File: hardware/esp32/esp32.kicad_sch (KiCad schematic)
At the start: 10 parts, among them J1 Conn_01x01, J2 Conn_01x02, J3 Conn_01x10, J6 Conn_01x01, U2 ESP32-S3-MINI-1-N8

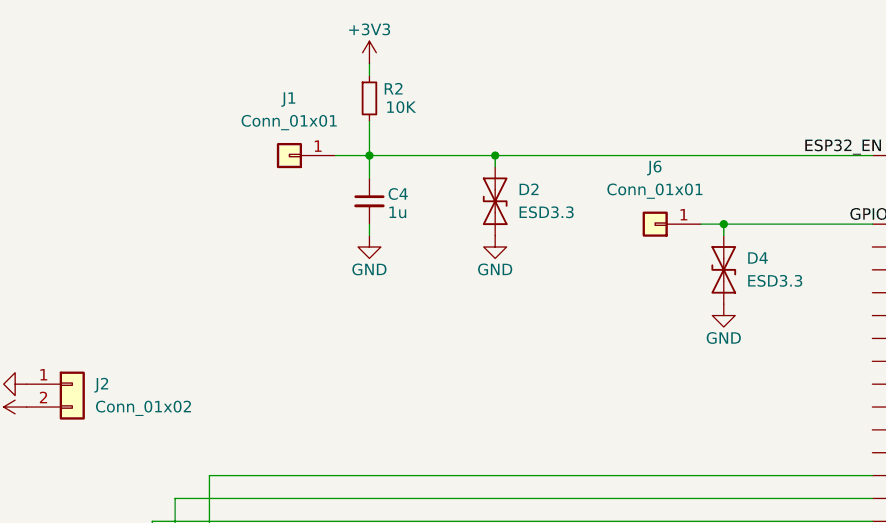
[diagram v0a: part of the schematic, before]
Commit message: wip esp32 v1
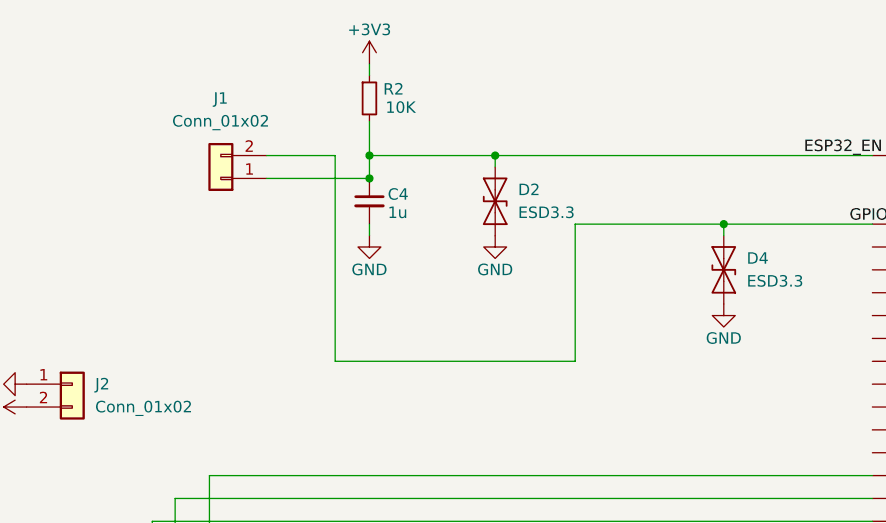
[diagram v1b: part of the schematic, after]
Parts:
- removed J1, J6: Conn_01x01, Connector_PinHeader_1.00mm:PinHeader_1x01_P1.00mm_Vertical, symbol Connector_Generic:Conn_01x01
- added J1: Conn_01x02, Connector_JST:JST_SH_BM02B-SRSS-TB_1x02-1MP_P1.00mm_Vertical, symbol Connector_Generic:Conn_01x02
- C18, C4: footprint Capacitor_SMD:C_0603_1608Metric -> Capacitor_SMD:C_0201_0603Metric
- R2: footprint Resistor_SMD:R_0402_1005Metric -> Resistor_SMD:R_0201_0603Metric
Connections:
- net ESP32_EN: now also J1.1 (Pin_1)
- net GPIO0: now also J1.2 (Pin_2)

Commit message: Revert "wip esp32 v1"
This reverts commit 4981c68ebba1a87f50308cda0493b3bcd30c48b4.
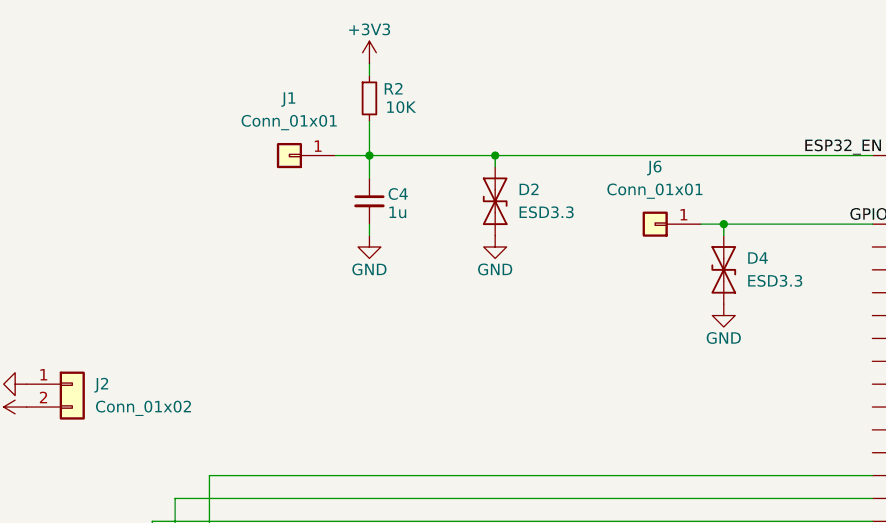
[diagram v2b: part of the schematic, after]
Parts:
- removed J1: Conn_01x02, Connector_JST:JST_SH_BM02B-SRSS-TB_1x02-1MP_P1.00mm_Vertical, symbol Connector_Generic:Conn_01x02
- added J1, J6: Conn_01x01, Connector_PinHeader_1.00mm:PinHeader_1x01_P1.00mm_Vertical, symbol Connector_Generic:Conn_01x01
- C18, C4: footprint Capacitor_SMD:C_0201_0603Metric -> Capacitor_SMD:C_0603_1608Metric
- R2: footprint Resistor_SMD:R_0201_0603Metric -> Resistor_SMD:R_0402_1005Metric
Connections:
- net ESP32_EN: now also J1.1 (Pin_1)
- net GPIO0: now also J6.1 (Pin_1)
